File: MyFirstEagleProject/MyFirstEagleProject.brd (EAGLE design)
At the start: 75.9 x 50.8 mm, 6 parts

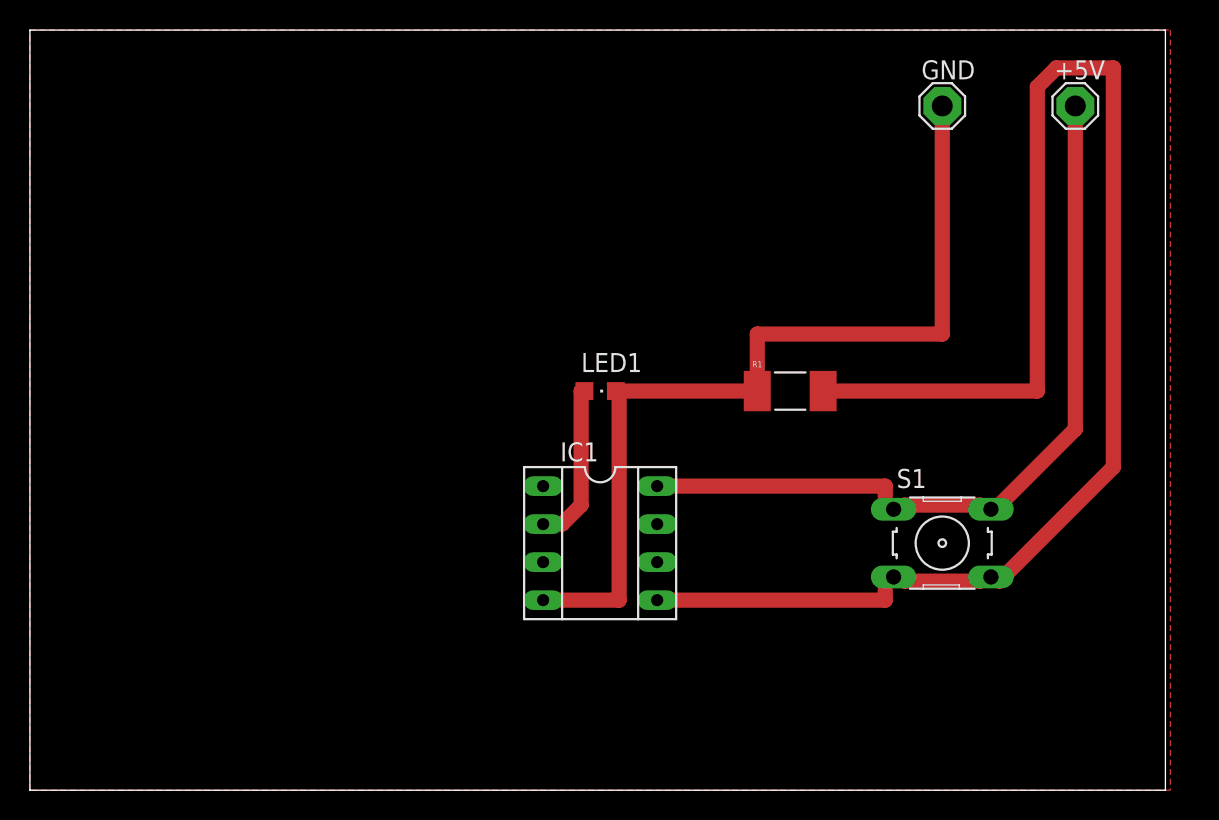
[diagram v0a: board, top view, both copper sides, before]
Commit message: Updated schematic/PCB files
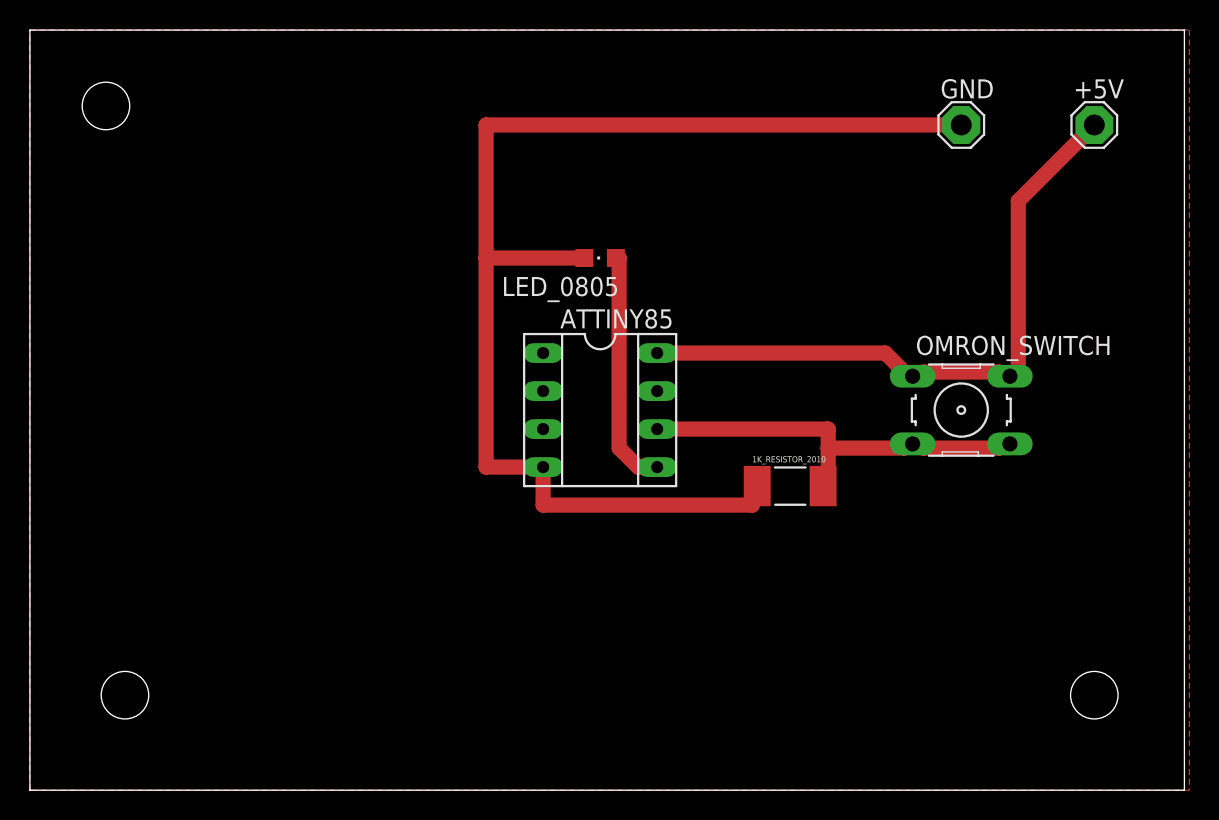
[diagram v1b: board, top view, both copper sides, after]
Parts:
- removed IC1: (no value), ic-package:SOCKET-08
- removed LED1: (no value), led:CHIPLED_0805
- removed R1: (no value), SparkFun:R2010
- removed S1: (no value), switch-omron:B3F-10XX
- added 1K_RESISTOR_2010: (no value), SparkFun:R2010
- added ATTINY85: (no value), ic-package:SOCKET-08
- added LED_0805: (no value), led:CHIPLED_0805
- added OMRON_SWITCH: (no value), switch-omron:B3F-10XX
- moved +5V 1.80 mm to (71.1, 44.5)
- moved GND 1.80 mm to (62.2, 44.5)
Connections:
- removed net N$3: IC1.2, LED1.A
- new net N$1: ATTINY85.5, LED_0805.A
- net 5V: now also ATTINY85.8, OMRON_SWITCH.1, OMRON_SWITCH.2; no longer IC1.8, S1.1, S1.2
- net GND: now also 1K_RESISTOR_2010.1, ATTINY85.4, LED_0805.C; no longer IC1.4, LED1.C, R1.1
- net N$6: now also 1K_RESISTOR_2010.2, ATTINY85.6, OMRON_SWITCH.3, OMRON_SWITCH.4; no longer IC1.5, R1.2, S1.3, S1.4
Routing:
- net N$6: track 102.1 -> 27.9 mm
- net GND: track 59.9 -> 82.8 mm
- net N$1: track 0.00 -> 16.0 mm
- net N$3: track 10.9 -> 0.00 mm
- net 5V: track 53.1 -> 43.5 mm
- added copper zone on layer 1, net N$2
- removed copper zone on layer 1, net N$1
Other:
- board size 75.9 x 50.8 mm -> 77.1 x 50.8 mm
